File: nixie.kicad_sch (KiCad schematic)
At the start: 15 parts, among them Q1 IRF840A, U1 UC3843_DIP8

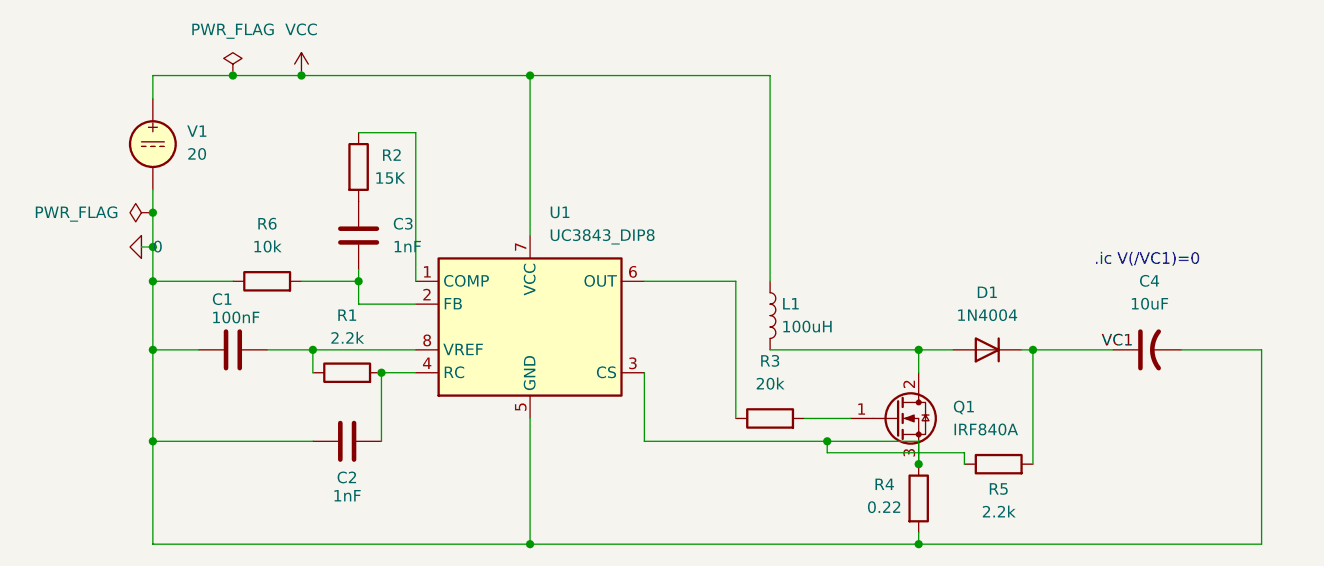
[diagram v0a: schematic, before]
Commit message: update
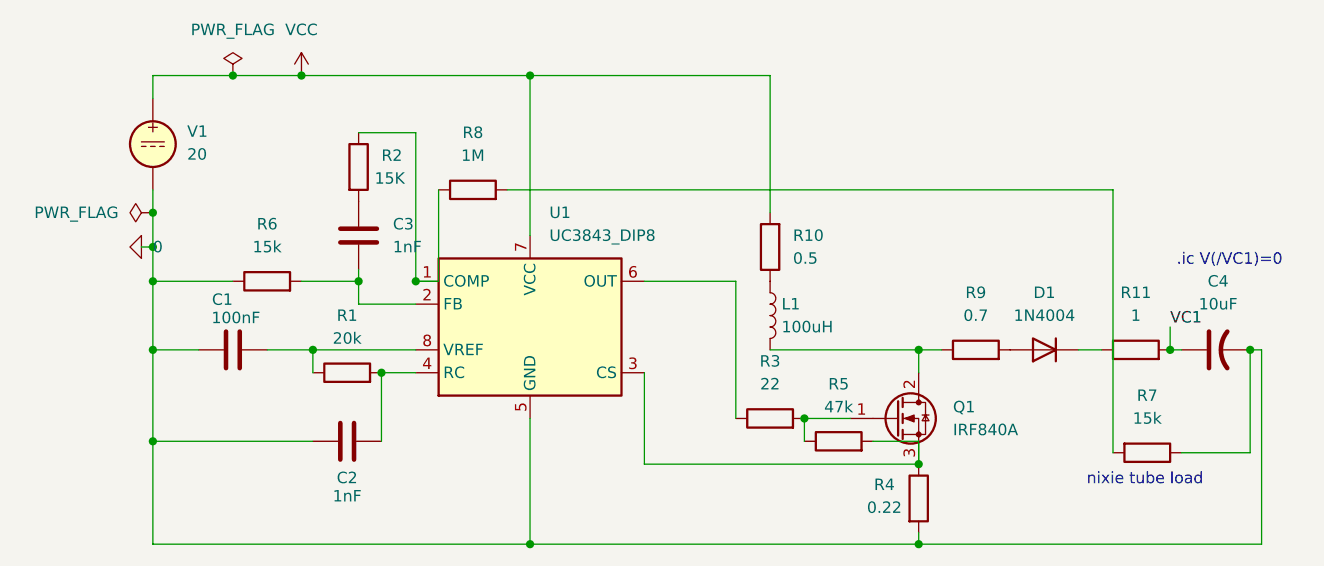
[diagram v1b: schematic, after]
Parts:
- added R10: 0.5, symbol Device:R
- added R11: 1, symbol Device:R
- added R7: 15k, symbol Device:R
- added R8: 1M, symbol Device:R
- added R9: 0.7, symbol Device:R
- R1: value 2.2k -> 20k
- R3: value 20k -> 22
- R5: value 2.2k -> 47k
- R6: value 10k -> 15k
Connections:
- net 0: now also R7.1
- net VC1: now also R11.2; no longer D1.1 (K), R5.2
- net VCC: now also R10.2; no longer L1.1
- net at R2.1, U1.1 (COMP): now also R8.1
- net at Q1.3 (S), R4.1, U1.3 (CS): now also R5.2; no longer R5.1
- net at L1.2, Q1.2 (D): now also R9.1; no longer D1.2 (A)
- net at Q1.1 (G), R3.2: now also R5.1
- new net: L1.1, R10.1
- new net: D1.1 (K), R11.1
- new net: D1.2 (A), R9.2
- new net: R7.2, R8.2
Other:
- note added: "nixie tube load"
- moved on the sheet: C4, D1
